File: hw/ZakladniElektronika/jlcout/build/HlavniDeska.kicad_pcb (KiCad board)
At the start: 4 copper layers, 100 x 70.5 mm, 149 parts, among them J11 Conn_01x40, J2 USB_C_Receptacle_USB2.0, J3 Conn_2Rows-75Pins, J4 Conn_01x07, J7 ESP-Programing_conector, J9 Conn_01x02, Q1 Q_NMOS_DGS-L, Q10 Q_PMOS_DGS-P, Q11 Q_NMOS_DGS-L, Q12 Q_NMOS_DGS-P, Q13 Q_PMOS_DGS-P, Q14 Q_NMOS_DGS-P, Q15 Q_NMOS_DGS-P, Q17 Q_NMOS_DGS-L, Q19 Q_NMOS_DGS-L, Q7 Q_PMOS_DGS-L, SW1 SW_Push, SW2 SW_Push, SW3 ON, SW4 BOOT, SW5 EN, U11 ESP32-S3-WROOM, U12 LD39200, U13 TPD4E02B04DQA, U15 TS3USB3031, U17 BateriCell_2x, U2 TXB0304RUT, U3 TPS61088RHLR, U4 AP33772, U5 TPD4E02B04DQA, U52 MCP1700x-180xxTT, U6 TXB0304RUT, U7 SL8261D-G3JE, U8 PCA9306DC, U9 BQ25895RTW

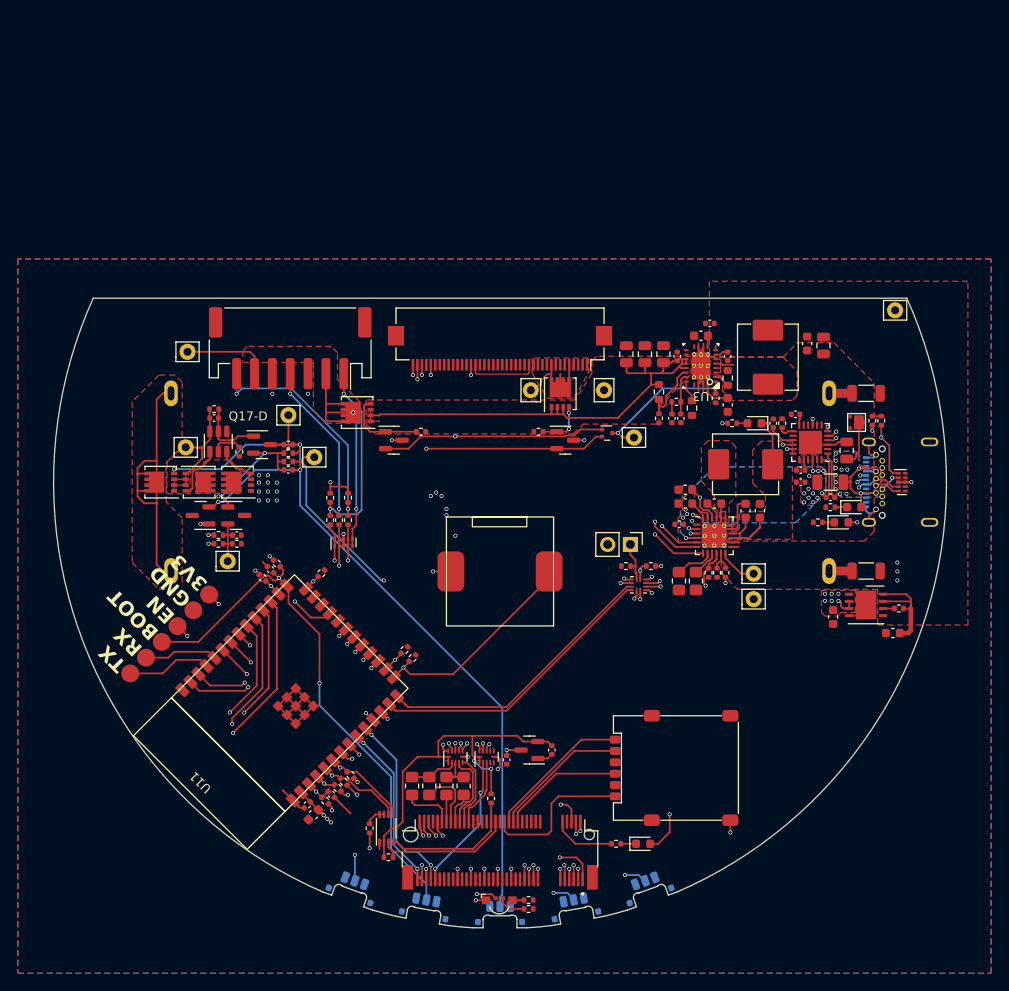
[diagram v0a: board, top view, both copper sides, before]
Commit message: Bordel Hw
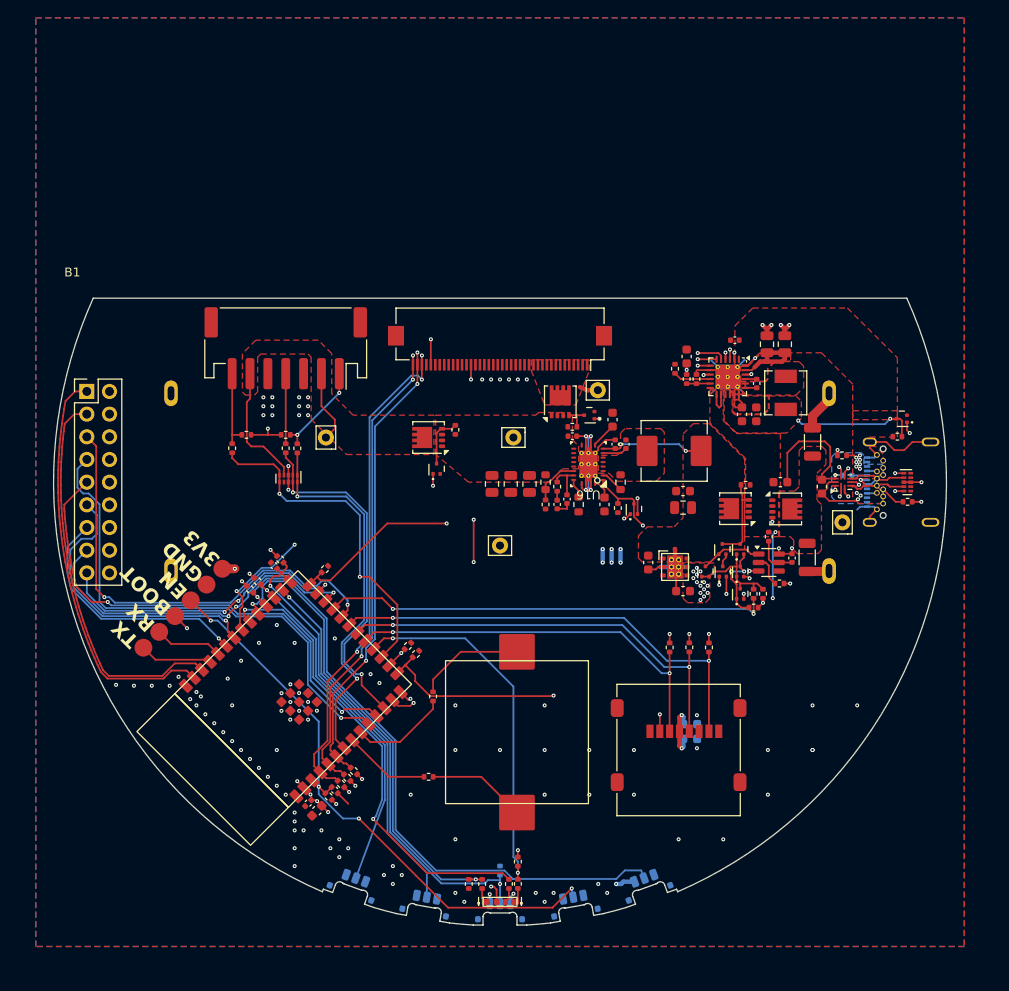
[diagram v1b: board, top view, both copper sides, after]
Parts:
- removed C138, C141, C163, C166: 1u, Capacitor_SMD:C_0402_1005Metric
- removed C139, C140: 100n, Capacitor_SMD:C_0402_1005Metric
- removed C164: 4.7u, Capacitor_SMD:C_0603_1608Metric
- removed C165: 47n, Capacitor_SMD:C_0603_1608Metric
- removed D121: LED_Dual_AKAK, RKL-LED:SMD,1.5x3.2mm 4pin
- removed D123: PTVSHC3N24, RKL-StandardPackages:DFN3-2x2
- removed F3, F4: 3A-6A, Inductor_SMD:L_1206_3216Metric
- removed J3: Conn_2Rows-75Pins, RKL-Connectors:Conn_M2
- removed J9: Conn_01x02, Connector_PinHeader_2.54mm:PinHeader_1x02_P2.54mm_Vertical
- removed L7: 2.2u, Inductor_SMD:L_Abracon_ASPI-0630LR
- removed LED3, LED4, LED5, LED6: red, LED_SMD:LED_0603_1608Metric
- removed Q10, Q13: Q_PMOS_DGS-P, Package_SON:Diodes_PowerDI3333-8
- removed Q11, Q17, Q19: Q_NMOS_DGS-L, Package_TO_SOT_SMD:SOT-23
- removed Q12, Q14, Q15: Q_NMOS_DGS-P, Package_SON:Diodes_PowerDI3333-8
- removed R18, R24, R25, R31: 4.7k, Resistor_SMD:R_0402_1005Metric
- removed R22, R23, R67, R70: 10k, Resistor_SMD:R_0402_1005Metric
- removed R27: 1k, Resistor_SMD:R_0402_1005Metric
- removed R33: 2k, Resistor_SMD:R_0402_1005Metric
- removed R42: 3.92k, Resistor_SMD:R_0402_1005Metric
- removed R43, R44: 150k, Resistor_SMD:R_0603_1608Metric
- removed R46: 56k, Resistor_SMD:R_0603_1608Metric
- removed R60: 200k, Resistor_SMD:R_0402_1005Metric
- removed R68: 1M, Resistor_SMD:R_0402_1005Metric
- removed R69: 200, Resistor_SMD:R_0402_1005Metric
- removed R71: 0, Resistor_SMD:R_0805_2012Metric_Pad1.20x1.40mm_HandSolder
- removed R72: 100, Resistor_SMD:R_0402_1005Metric
- removed TP2: TestPoint-BAT, Connector_Pin:Pin_D0.9mm_L10.0mm_W2.4mm_FlatFork
- removed TP3: TestPoint-VCC, Connector_Pin:Pin_D0.9mm_L10.0mm_W2.4mm_FlatFork
- removed TP4: TestPoint-BUTTON_ON, Connector_Pin:Pin_D0.9mm_L10.0mm_W2.4mm_FlatFork
- removed TP5: TestPoint-EN_ALL, Connector_Pin:Pin_D0.9mm_L10.0mm_W2.4mm_FlatFork
- removed TP6: TestPoint-Charger_QON, Connector_Pin:Pin_D0.9mm_L10.0mm_W2.4mm_FlatFork
- removed TP7: TestPoint-Charger_ILIM, Connector_Pin:Pin_D0.9mm_L10.0mm_W2.4mm_FlatFork
- removed U17: BateriCell_2x, RKL-Batteries:battery_dock
- removed U4: AP33772, Package_DFN_QFN:QFN-24-1EP_4x4mm_P0.5mm_EP2.6x2.6mm
- removed U52: MCP1700x-180xxTT, Package_TO_SOT_SMD:SOT-23
- removed U53: ~, RKL-Connectors:SMN-305-ARP7
- removed U6: TXB0304RUT, Package_DFN_QFN:Texas_R-PUQFN-N12
- added B1: HlavniDeska, RKL-AuxiliarySymbols:Board, F.Cu at (164.5, 69.4)
- added C158: 100p, Capacitor_SMD:C_0402_1005Metric, F.Cu at (217.5, 91.9)
- added C161: 10u, Capacitor_SMD:C_0603_1608Metric, F.Cu at (237.1, 82.4)
- added C162: 10u, Capacitor_SMD:C_0603_1608Metric, F.Cu at (246.1, 90.5)
- added D125: LED_ARGB, RKL-LED:XL-3806RGBC-4L, F.Cu at (210.0, 137.0)
- added F1: 3A-6A, Inductor_SMD:L_1206_3216Metric, F.Cu at (245.0, 85.5)
- added F2: 3A-6A, Inductor_SMD:L_1206_3216Metric, F.Cu at (244.4, 98.4)
- added J1: Conn_02x09_Counter_Clockwise, Connector_PinHeader_2.54mm:PinHeader_2x09_P2.54mm_Vertical, F.Cu at (163.7, 79.8)
- added J5: Micro_SD_Card, Connector_Card:microSD_HC_Molex_47219-2001, F.Cu at (230.0, 120.0)
- added L5: 1.2u, Inductor_SMD:L_Abracon_ASPI-0630LR, F.Cu at (229.5, 86.5)
- added Q2: NMOS, Package_TO_SOT_SMD:SOT-723, F.Cu at (220.0, 82.5)
- added Q28: NMOS, Package_TO_SOT_SMD:SOT-723, F.Cu at (234.9, 100.0)
- added Q4: NMOS, Package_TO_SOT_SMD:SOT-723, F.Cu at (233.0, 100.0)
- added Q5: NMOS, Package_TO_SOT_SMD:SOT-723, F.Cu at (234.9, 97.5)
- added Q6: NMOS, Package_TO_SOT_SMD:SOT-723, F.Cu at (236.9, 97.5)
- added Q8: NMOS, Package_TO_SOT_SMD:SOT-723, F.Cu at (236.9, 102.5)
- added Q9: NMOS, Package_TO_SOT_SMD:SOT-723, F.Cu at (255.0, 82.9)
- added R34: 2k, Resistor_SMD:R_0402_1005Metric, F.Cu at (241.3, 101.3)
- added R40: 100k, Resistor_SMD:R_0402_1005Metric, F.Cu at (237.5, 90.3)
- added R51: 10k, Resistor_SMD:R_0402_1005Metric, F.Cu at (239.4, 102.5)
- added R52: 200, Resistor_SMD:R_0402_1005Metric, F.Cu at (238.4, 102.5)
- added R53: 200k, Resistor_SMD:R_0402_1005Metric, F.Cu at (254.5, 84.9)
- added R54: 150k, Resistor_SMD:R_0603_1608Metric, F.Cu at (223.5, 90.0)
- added R55: 150k, Resistor_SMD:R_0603_1608Metric, F.Cu at (218.8, 92.5)
- added R56: 3.92k, Resistor_SMD:R_0402_1005Metric, F.Cu at (216.4, 90.5)
- added R57: 56k, Resistor_SMD:R_0603_1608Metric, F.Cu at (215.1, 90.0)
- added R58: 17.4k, Resistor_SMD:R_0402_1005Metric, F.Cu at (215.1, 92.5)
- added R79: 10k, Resistor_SMD:R_0402_1005Metric, B.Cu at (210.0, 133.5)
- added U10: NCP708, RKL-StandardPackages:UDFN6-3x3mm, F.Cu at (229.6, 99.5)
- added U14: BateriCell_2x, RKL-Batteries:battery_dock, B.Cu at (210.0, 90.0)
- added U16: TPS61088RHLR, RKL-StandardPackages:RHL0020A, F.Cu at (219.9, 88.0)
- BZ1: footprint RKL-StandardPackages:PKLCS1212E-(RH-Logic_piezzo) -> RKL-Audio:ELKS-PIEZO
- C136: value 10u -> 10uF; footprint Capacitor_SMD:C_0805_2012Metric -> Capacitor_SMD:C_0603_1608Metric; moved to B.Cu
- C137: value 100n -> 10uF; footprint Capacitor_SMD:C_0402_1005Metric -> Capacitor_SMD:C_0603_1608Metric; moved to B.Cu
- C142: value 1u -> 22u; footprint Capacitor_SMD:C_0402_1005Metric -> Capacitor_SMD:C_0805_2012Metric
- C143: value 100n -> 10u; footprint Capacitor_SMD:C_0402_1005Metric -> Capacitor_SMD:C_0603_1608Metric
- C144, C148: value 1u -> 100n
- C145, C155: value 10u -> 4.7u
- C146: value 10u -> 100n; footprint Capacitor_SMD:C_0603_1608Metric -> Capacitor_SMD:C_0402_1005Metric
- C147: value 10u -> 22u; footprint Capacitor_SMD:C_0603_1608Metric -> Capacitor_SMD:C_0805_2012Metric
- C150: value 4.7u -> 47n
- C151: value 100n -> 22u; footprint Capacitor_SMD:C_0402_1005Metric -> Capacitor_SMD:C_0805_2012Metric
- C152: value 47n -> 10u
- C154: value 4.7u -> 22u; footprint Capacitor_SMD:C_0603_1608Metric -> Capacitor_SMD:C_0805_2012Metric
- C159: value 22u -> 10u; footprint Capacitor_SMD:C_0805_2012Metric -> Capacitor_SMD:C_0603_1608Metric
- C160: value 100p -> 10u; footprint Capacitor_SMD:C_0402_1005Metric -> Capacitor_SMD:C_0603_1608Metric
- C5: value 22u -> 1u; footprint Capacitor_SMD:C_0805_2012Metric -> Capacitor_SMD:C_0402_1005Metric
- C6: value 10u -> 47n; footprint Capacitor_SMD:C_0603_1608Metric -> Capacitor_SMD:C_0402_1005Metric
- C7: value 100n -> 4.7u; footprint Capacitor_SMD:C_0402_1005Metric -> Capacitor_SMD:C_0603_1608Metric
- L6: value 1.2u -> 0.47u; footprint Inductor_SMD:L_Abracon_ASPI-0630LR -> Inductor_SMD:L_Sunlord_MWSA0402S
- Q1: value Q_NMOS_DGS-L -> NMOS; footprint Package_TO_SOT_SMD:SOT-23 -> Package_TO_SOT_SMD:SOT-723
- Q7: value Q_PMOS_DGS-L -> NMOS; footprint Package_TO_SOT_SMD:SOT-23 -> Package_TO_SOT_SMD:SOT-723
- R11: value 10m -> 1k; footprint Resistor_SMD:R_1206_3216Metric -> Resistor_SMD:R_0402_1005Metric
- R13: value 4.7k -> 10k
- R14: value 0-nc -> 330; footprint Resistor_SMD:R_0805_2012Metric_Pad1.20x1.40mm_HandSolder -> Resistor_SMD:R_0402_1005Metric
- R15: value 0 -> 330; footprint Resistor_SMD:R_0805_2012Metric_Pad1.20x1.40mm_HandSolder -> Resistor_SMD:R_0402_1005Metric
- R16: value 0-nc -> 10k; footprint Resistor_SMD:R_0805_2012Metric_Pad1.20x1.40mm_HandSolder -> Resistor_SMD:R_0402_1005Metric
- R17: value 0 -> 10k; footprint Resistor_SMD:R_0805_2012Metric_Pad1.20x1.40mm_HandSolder -> Resistor_SMD:R_0402_1005Metric
- R19: value 10k -> 150
- R2, R41: value 200k -> 10k
- R20: value 10k -> 56k
- R21: value 0 -> 100k; footprint Resistor_SMD:R_0805_2012Metric_Pad1.20x1.40mm_HandSolder -> Resistor_SMD:R_0402_1005Metric
- R26: value 200k -> 470
- R35: value 470 -> 10k
- R36: value 1M -> 10k
- R4: moved to B.Cu
- R47: value 17.4k -> 200k
- R5: value 4.7k -> 1k
- R50: value 200k -> 17.4k
- TP1: value TestPoint-Q16_G -> TestPoint-5V_A
- U12: value LD39200 -> SL8261D-G3JE; footprint Package_DFN_QFN:DFN-8-1EP_4x4mm_P0.8mm_EP2.3x3.24mm -> Package_TO_SOT_SMD:SOT-23-6
- U15: value TS3USB3031 -> WSD20L75DN33; footprint Package_DFN_QFN:Texas_X2QFN-12_1.6x1.6mm_P0.4mm -> Package_SON:Diodes_PowerDI3333-8
- U2: value TXB0304RUT -> BL1530TQFN; footprint Package_DFN_QFN:Texas_R-PUQFN-N12 -> Package_DFN_QFN:UQFN-10_1.4x1.8mm_P0.4mm
- U3: value TPS61088RHLR -> BQ25895M; footprint RKL-StandardPackages:RHL0020A -> Package_DFN_QFN:Texas_RTW_WQFN-24-1EP_4x4mm_P0.5mm_EP2.7x2.7mm_ThermalVias
- U7: value SL8261D-G3JE -> WSD20L75DN33; footprint Package_TO_SOT_SMD:SOT-23-6 -> Package_SON:Diodes_PowerDI3333-8
- U8: value PCA9306DC -> WSD20L75DN33; footprint Package_SO:VSSOP-8_2.3x2mm_P0.5mm -> Package_SON:Diodes_PowerDI3333-8
- U9: value BQ25895RTW -> WSD20L75DN33; footprint Package_DFN_QFN:Texas_S-PWQFN-N24_EP2.7x2.7mm_ThermalVias -> Package_SON:Diodes_PowerDI3333-8
- moved R2 67.4 mm to (248.3, 87.0), turned to 180 degrees
- moved U7 64.0 mm to (242.0, 93.0), turned to 0 degrees
- moved TP1 63.2 mm to (248.3, 94.5), turned to 90 degrees
- moved R12 62.4 mm to (206.5, 135.0)
- moved R11 59.5 mm to (208.0, 135.0), turned to 90 degrees
- moved R36 59.5 mm to (231.2, 108.5), turned to -90 degrees
- moved C144 57.3 mm to (242.7, 98.5), turned to 90 degrees
- moved R5 55.5 mm to (211.0, 135.0), turned to 90 degrees
- moved Q7 55.4 mm to (236.9, 100.0), turned to 90 degrees
- moved R26 54.5 mm to (240.1, 96.1), turned to -90 degrees
- moved U2 53.2 mm to (248.4, 90.0)
- moved C143 53.2 mm to (230.5, 91.0)
- moved U8 53.0 mm to (236.4, 93.0), turned to 180 degrees
- moved R35 52.3 mm to (233.4, 108.5), turned to -90 degrees
- moved R13 50.7 mm to (212.0, 132.5), turned to -90 degrees
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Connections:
- BZ1 pad 1: /HlavniDeska/ESP32S3/IO03-PD -> Net-(BZ1--)
- BZ1 pad 2: /HlavniDeska/ESP32S3/IO01 -> Net-(BZ1-+)
- C136 pad 1: /HlavniDeska/USB/V_USB -> /HlavniDeska/3V3
- C137 pad 1: /HlavniDeska/USB/V_USB -> /HlavniDeska/3V3
- C137 pad 2: /HlavniDeska/SpravceNapajeni/VBUS -> GND
- C142 pad 1: /HlavniDeska/SpravceNapajeni/5V-IN -> /HlavniDeska/SpravceNapajeni/Power multiplier/VCC
- C143 pad 1: Net-(Q7-D) -> /HlavniDeska/SpravceNapajeni/Power multiplier/VCC
- C143 pad 2: Net-(U7-GND) -> GND
- C144 pad 1: Net-(Q17-D) -> Net-(U12-VCC)
- C144 pad 2: Net-(Q19-G) -> GND
- C145 pad 1: Net-(LED5-K) -> /HlavniDeska/SpravceNapajeni/Power multiplier/VCC
- C146 pad 1: Net-(LED5-K) -> /HlavniDeska/SpravceNapajeni/Power multiplier/VCC
- C147 pad 1: Net-(U9-PMID) -> Net-(U3-PMID)
- C148 pad 1: /HlavniDeska/GPSKomunikacniModul/1V8 -> SW
- C148 pad 2: GND -> Net-(U16-BOOT)
- C149 pad 1: /HlavniDeska/3V3 -> /HlavniDeska/SpravceNapajeni/5V-IN
- C150 pad 1: VCC -> Net-(U16-SS)
- C151 pad 1: SW -> Net-(U3-PMID)
- C151 pad 2: Net-(U3-BOOT) -> GND
- C152 pad 1: Net-(U3-SS) -> /HlavniDeska/3V3
- C154 pad 1: Net-(U3-VCC) -> /HlavniDeska/SpravceNapajeni/5V-IN
- C155 pad 1: /HlavniDeska/3V3 -> Net-(U16-VCC)
- C159 pad 1: /HlavniDeska/SpravceNapajeni/5V-IN -> /HlavniDeska/SpravceNapajeni/Charging/BATT
- C160 pad 1: Net-(U3-COMP) -> /HlavniDeska/SpravceNapajeni/Charging/SYS
- C5 pad 1: VCC -> /HlavniDeska/USB/V_USB
- C6 pad 1: VCC -> /HlavniDeska/SpravceNapajeni/Charging/SW
- C6 pad 2: GND -> Net-(U3-BTST)
- C7 pad 1: VCC -> Net-(U3-REGN)
- D122 pad 3: /HlavniDeska/SpravceNapajeni/NapajeciRozcesti/EN-5V -> /HlavniDeska/SpravceNapajeni/Power multiplier/EN-5V
- J2 pad A6: /HlavniDeska/C.D+ -> /HlavniDeska/USB/D+
- J2 pad A7: /HlavniDeska/C.D- -> /HlavniDeska/USB/D-
- J2 pad B6: /HlavniDeska/C.D+ -> /HlavniDeska/USB/D+
- J2 pad B7: /HlavniDeska/C.D- -> /HlavniDeska/USB/D-
- L6 pad 1: VCC -> /HlavniDeska/SpravceNapajeni/Charging/SW
- L6 pad 2: SW -> /HlavniDeska/SpravceNapajeni/Charging/SYS
- Q1 pad 1: Net-(Q1-D) -> /HlavniDeska/ESP32S3/IO46-PD
- Q1 pad 2: /HlavniDeska/ESP32S3/IO46-PD -> GND
- Q1 pad 3: GND -> Net-(Q1-D)
- Q7 pad 1: Net-(Q7-D) -> Net-(Q4-G)
- Q7 pad 2: Net-(Q17-D) -> GND
- Q7 pad 3: Net-(Q7-S) -> Net-(Q6-S)
- R11 pad 1: /HlavniDeska/USB/V_USB -> Net-(D125-RK)
- R11 pad 2: /HlavniDeska/SpravceNapajeni/VBUS -> /HlavniDeska/ESP32S3/IO38
- R12 pad 1: GND -> /HlavniDeska/ESP32S3/IO38
- R12 pad 2: Net-(U4-OTP) -> GND
- R13 pad 1: GND -> /HlavniDeska/SpravceNapajeni/CHARGER_STAT
- R13 pad 2: Net-(LED4-K) -> /HlavniDeska/ESP32S3/IO10
- R14 pad 1: /HlavniDeska/GPSKomunikacniModul/UART_RXD(I)(1.8V) -> /HlavniDeska/ESP32S3/IO15
- R14 pad 2: Net-(J3-Pin_58) -> Net-(BZ1--)
- R15 pad 1: /HlavniDeska/GPSKomunikacniModul/UART_RXD(I)(1.8V) -> /HlavniDeska/ESP32S3/IO16
- R15 pad 2: Net-(J3-Pin_62) -> Net-(BZ1-+)
- R16 pad 1: /HlavniDeska/GPSKomunikacniModul/UART_TXD(O)(1.8V) -> /HlavniDeska/3V3
- R16 pad 2: Net-(J3-Pin_60) -> /HlavniDeska/ESP32S3/IO36
- R17 pad 1: /HlavniDeska/GPSKomunikacniModul/UART_TXD(O)(1.8V) -> /HlavniDeska/3V3
- R17 pad 2: Net-(J3-Pin_64) -> /HlavniDeska/ESP32S3/IO37
- R19 pad 1: Net-(U9-TS) -> Net-(U3-ILIM)
- R2 pad 1: /HlavniDeska/3V3 -> /HlavniDeska/USB/V_USB
- R2 pad 2: Net-(U8-EN) -> /HlavniDeska/SpravceNapajeni/USB_SEL
- R20 pad 1: Net-(U9-TS) -> Net-(U3-REGN)
- R20 pad 2: Net-(U9-REGN) -> Net-(U3-TS)
- R21 pad 2: Net-(U9-OTG) -> Net-(U3-TS)
- R26 pad 1: Net-(Q17-D) -> /HlavniDeska/SpravceNapajeni/Charging/BATT
- R26 pad 2: Net-(Q19-G) -> Net-(U12-VCC)
- R28 pad 1: GND -> Net-(D125-BK)
- R28 pad 2: Net-(D121-K1) -> /HlavniDeska/ESP32S3/IO10
- R29 pad 2: /HlavniDeska/ESP32S3/IO41 -> /HlavniDeska/ESP32S3/IO07
- R30 pad 2: /HlavniDeska/ESP32S3/IO42 -> /HlavniDeska/ESP32S3/IO08
- R32 pad 2: Net-(Q11-D) -> Net-(Q2-D)
- R35 pad 1: VCC -> /HlavniDeska/3V3
- R35 pad 2: Net-(Q7-S) -> /HlavniDeska/ESP32S3/IO13
- R36 pad 1: Net-(U7-GND) -> /HlavniDeska/3V3
- R36 pad 2: Net-(Q7-D) -> /HlavniDeska/ESP32S3/IO12
- R41 pad 1: GND -> /HlavniDeska/3V3
- R41 pad 2: /HlavniDeska/SpravceNapajeni/NapajeciRozcesti/EN-5V -> /HlavniDeska/ESP32S3/IO11
- R47 pad 2: Net-(U3-FB) -> /HlavniDeska/SpravceNapajeni/Power multiplier/EN-5V
- R49 pad 2: /HlavniDeska/ESP32S3/IO02 -> /HlavniDeska/ESP32S3/IO09
- R5 pad 1: GND -> Net-(D125-GK)
- R5 pad 2: Net-(LED3-K) -> /HlavniDeska/ESP32S3/IO39
- R50 pad 1: VCC -> Net-(Q6-S)
- R50 pad 2: Net-(U12-EN) -> /HlavniDeska/3V3
- SW3 pad 1: GND -> /HlavniDeska/SpravceNapajeni/Charging/BATT
- SW3 pad 2: Net-(Q19-G) -> /HlavniDeska/ESP32S3/IO35
- TP1 pad 1: Net-(Q17-D) -> /HlavniDeska/USB/V_USB
- TP8 pad 1: /HlavniDeska/SpravceNapajeni/NapajeciRozcesti/EN-5V -> /HlavniDeska/SpravceNapajeni/Power multiplier/EN-5V
- U11 pad 17: /HlavniDeska/KM_DTR -> /HlavniDeska/ESP32S3/IO09
- U11 pad 18: /HlavniDeska/KM_RTS -> /HlavniDeska/ESP32S3/IO10
- U11 pad 19: /HlavniDeska/KM_CST -> /HlavniDeska/ESP32S3/IO11
- U11 pad 20: /HlavniDeska/KM_RXD -> /HlavniDeska/ESP32S3/IO12
- U11 pad 21: /HlavniDeska/KM_TXD -> /HlavniDeska/ESP32S3/IO13
- U12 pad 1: /HlavniDeska/3V3 -> Net-(Q4-D)
- U12 pad 2: /HlavniDeska/3V3 -> Net-(U12-VM)
- U12 pad 3: /HlavniDeska/3V3 -> Net-(Q9-G)
- U12 pad 4: GND -> unconnected-(U12-TD-Pad4)
- U12 pad 5: unconnected-(U12-PG-Pad5) -> Net-(U12-VCC)
- U12 pad 6: Net-(U12-EN) -> GND
- U13 pad 1: /HlavniDeska/USB/USB_CC1 -> /HlavniDeska/USB/V_USB
- U13 pad 2: /HlavniDeska/USB/USB_CC2 -> /HlavniDeska/USB/D-
- U13 pad 4: /HlavniDeska/C.D- -> /HlavniDeska/USB/D+
- U13 pad 5: /HlavniDeska/C.D+ -> /HlavniDeska/USB/V_USB
- U15 pad 1: /HlavniDeska/SpravceNapajeni/DSEL -> /HlavniDeska/SpravceNapajeni/5V-IN
- U15 pad 2: Net-(J9-Pin_1) -> /HlavniDeska/SpravceNapajeni/5V-IN
- U15 pad 3: /HlavniDeska/Nabijecka.D+ -> /HlavniDeska/SpravceNapajeni/5V-IN
- U15 pad 4: /HlavniDeska/Nabijecka.D- -> Net-(Q2-D)
- U15 pad 5: /HlavniDeska/ESP.D+ -> /HlavniDeska/5V-OUT
- U2 pad 1: /HlavniDeska/GPSKomunikacniModul/1V8 -> /HlavniDeska/Nabijecka.D+
- U2 pad 10: /HlavniDeska/KM_TXD -> /HlavniDeska/SpravceNapajeni/USB_SEL
- U2 pad 2: /HlavniDeska/GPSKomunikacniModul/UART_TXD(O)(1.8V) -> /HlavniDeska/ESP.D+
- U2 pad 3: /HlavniDeska/GPSKomunikacniModul/UART_RXD(I)(1.8V) -> /HlavniDeska/USB/D+
- U2 pad 4: /HlavniDeska/GPSKomunikacniModul/UART_CTS(O)(1.8V) -> GND
- U2 pad 5: /HlavniDeska/GPSKomunikacniModul/UART_RTS(I)(1.8V) -> /HlavniDeska/USB/D-
- U2 pad 6: GND -> /HlavniDeska/ESP.D-
- U2 pad 7: /HlavniDeska/KM_RTS -> /HlavniDeska/Nabijecka.D-
- U2 pad 8: /HlavniDeska/KM_CST -> GND
- U2 pad 9: /HlavniDeska/KM_RXD -> /HlavniDeska/USB/V_USB
- U3 pad 1: Net-(U3-VCC) -> /HlavniDeska/USB/V_USB
- U3 pad 10: Net-(U3-SS) -> Net-(U3-ILIM)
- U3 pad 11: unconnected-(U3-NC-Pad11) -> Net-(U3-TS)
- U3 pad 13: unconnected-(U3-MODE-Pad13) -> /HlavniDeska/SpravceNapajeni/Charging/BATT
- U3 pad 14: /HlavniDeska/SpravceNapajeni/5V-IN -> /HlavniDeska/SpravceNapajeni/Charging/BATT
- U3 pad 15: /HlavniDeska/SpravceNapajeni/5V-IN -> /HlavniDeska/SpravceNapajeni/Charging/SYS
- U3 pad 16: /HlavniDeska/SpravceNapajeni/5V-IN -> /HlavniDeska/SpravceNapajeni/Charging/SYS
- U3 pad 17: Net-(U3-FB) -> GND
- U3 pad 18: Net-(U3-COMP) -> GND
- U3 pad 19: Net-(U3-ILIM) -> /HlavniDeska/SpravceNapajeni/Charging/SW
- U3 pad 2: /HlavniDeska/SpravceNapajeni/NapajeciRozcesti/EN-5V -> /HlavniDeska/Nabijecka.D+
- U3 pad 20: GND -> /HlavniDeska/SpravceNapajeni/Charging/SW
- U3 pad 21: GND -> Net-(U3-BTST)
- U3 pad 3: Net-(U3-FSW) -> /HlavniDeska/Nabijecka.D-
- U3 pad 4: SW -> /HlavniDeska/SpravceNapajeni/CHARGER_STAT
- U3 pad 5: SW -> /HlavniDeska/SCL
- U3 pad 6: SW -> /HlavniDeska/SDA
- U3 pad 7: SW -> /HlavniDeska/INT
- U3 pad 8: Net-(U3-BOOT) -> GND
- U3 pad 9: VCC -> /HlavniDeska/SpravceNapajeni/Charging/CE
- U5 pad 1: /HlavniDeska/ESP32S3/IO41 -> /HlavniDeska/ESP32S3/IO07
- U5 pad 10: /HlavniDeska/ESP32S3/IO41 -> /HlavniDeska/ESP32S3/IO07
- U5 pad 2: /HlavniDeska/ESP32S3/IO42 -> /HlavniDeska/ESP32S3/IO08
- U5 pad 4: /HlavniDeska/ESP32S3/IO02 -> /HlavniDeska/ModulovyKonektor/5V
- U5 pad 5: /HlavniDeska/ModulovyKonektor/5V -> /HlavniDeska/ESP32S3/IO09
- U5 pad 6: /HlavniDeska/ModulovyKonektor/5V -> /HlavniDeska/ESP32S3/IO09
- U5 pad 7: /HlavniDeska/ESP32S3/IO02 -> unconnected-(U5-NC-Pad7)
- U5 pad 9: /HlavniDeska/ESP32S3/IO42 -> /HlavniDeska/ESP32S3/IO08
- U7 pad 1: Net-(Q15-G) -> /HlavniDeska/SpravceNapajeni/Charging/BATT
- U7 pad 2: Net-(U7-VM) -> /HlavniDeska/SpravceNapajeni/Charging/BATT
- U7 pad 3: Net-(Q14-G) -> /HlavniDeska/SpravceNapajeni/Charging/BATT
- U7 pad 4: unconnected-(U7-TD-Pad4) -> GND
- U7 pad 5: Net-(Q7-D) -> Net-(U7-D)
- U8 pad 1: GND -> /HlavniDeska/SpravceNapajeni/Charging/BATT
- U8 pad 2: /HlavniDeska/GPSKomunikacniModul/1V8 -> /HlavniDeska/SpravceNapajeni/Charging/BATT
- U8 pad 3: /HlavniDeska/GPSKomunikacniModul/SCL(1.8V) -> /HlavniDeska/SpravceNapajeni/Charging/BATT
- U8 pad 4: /HlavniDeska/GPSKomunikacniModul/SDA(1.8V) -> Net-(Q5-D)
- U8 pad 5: /HlavniDeska/SDA -> /HlavniDeska/SpravceNapajeni/Power multiplier/VCC
- U9 pad 1: /HlavniDeska/SpravceNapajeni/VBUS -> /HlavniDeska/SpravceNapajeni/5V-IN
- U9 pad 2: /HlavniDeska/Nabijecka.D+ -> /HlavniDeska/SpravceNapajeni/5V-IN
- U9 pad 3: /HlavniDeska/Nabijecka.D- -> /HlavniDeska/SpravceNapajeni/5V-IN
- U9 pad 4: /HlavniDeska/SpravceNapajeni/Nabijecka/STAT -> Net-(Q1-D)
- U9 pad 5: /HlavniDeska/SCL -> /HlavniDeska/ModulovyKonektor/5V
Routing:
- net VCC: track 172.4 -> 0.00 mm, vias 11 -> 0
- net /HlavniDeska/SpravceNapajeni/CHARGER_STAT: track 0.00 -> 100.0 mm, vias 0 -> 2
- net /HlavniDeska/ESP32S3/IO35: track 16.0 -> 110.5 mm, vias 2 -> 3
- net Net-(Q19-G): track 74.7 -> 0.00 mm, vias 2 -> 0
- net /HlavniDeska/SpravceNapajeni/Charging/BATT: track 0.00 -> 68.7 mm, vias 0 -> 4
- net /HlavniDeska/INT: track 145.0 -> 88.6 mm, vias 6 -> 4
- net /HlavniDeska/SpravceNapajeni/5V-IN: track 55.5 -> 0.04 mm
- net /HlavniDeska/ESP32S3/IO14: track 0.00 -> 52.1 mm, vias 0 -> 2
- net /HlavniDeska/ESP32S3/IO13: track 0.00 -> 51.5 mm, vias 0 -> 2
- net /HlavniDeska/ESP32S3/IO12: track 0.00 -> 48.4 mm, vias 0 -> 2
- net /HlavniDeska/ESP32S3/IO11: track 0.00 -> 45.3 mm, vias 0 -> 2
- net GND: track 95.9 -> 137.9 mm, vias 32 -> 113
- net /HlavniDeska/GPSKomunikacniModul/1V8: track 41.5 -> 0.00 mm, vias 2 -> 0
- net /HlavniDeska/ESP32S3/IO10: track 0.00 -> 40.9 mm, vias 0 -> 2
- net /HlavniDeska/ESP32S3/IO47: track 0.00 -> 39.3 mm, vias 0 -> 3
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- added copper zone on F.Cu, net /HlavniDeska/SpravceNapajeni/Charging/BATT
- added copper zone on F.Cu, net /HlavniDeska/SpravceNapajeni/Charging/SW
- added copper zone on F.Cu, net /HlavniDeska/SpravceNapajeni/Charging/SYS
- added copper zone on F.Cu, net /HlavniDeska/SpravceNapajeni/Power multiplier/VCC
- added copper zone on F.Cu, net Net-(U3-PMID)
- added copper zone on F.Cu, net Net-(U7-D)
- removed copper zone on B.Cu, net /HlavniDeska/SpravceNapajeni/VBUS
- removed copper zone on F.Cu, net /HlavniDeska/SpravceNapajeni/VBUS
- removed copper zone on F.Cu, net Net-(C165-Pad1)
- removed copper zone on F.Cu, net Net-(LED5-K)
- removed copper zone on F.Cu, net Net-(Q12-D)
- removed copper zone on F.Cu, net Net-(Q14-D)
- removed copper zone on F.Cu, net Net-(U7-GND)
- removed copper zone on F.Cu, net VCC
- removed copper zone on In1.Cu, net VCC
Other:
- board size 100 x 70.5 mm -> 100 x 70.2 mm
- board text removed: "Q17-D"
